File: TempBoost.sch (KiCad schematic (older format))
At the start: 63 parts, among them J1 Conn_01x02, J2 Conn_01x02, Q201 Q_NMOS_GSD, SW101 SW_SPST, T101 3FD-224, U101 DF005S2, U201 MIC2920, U203 UCC27517A, U204 2925, U205 LM2904, U206 TPS1H100, U207 LM1117-5.0, U208 MAX4477

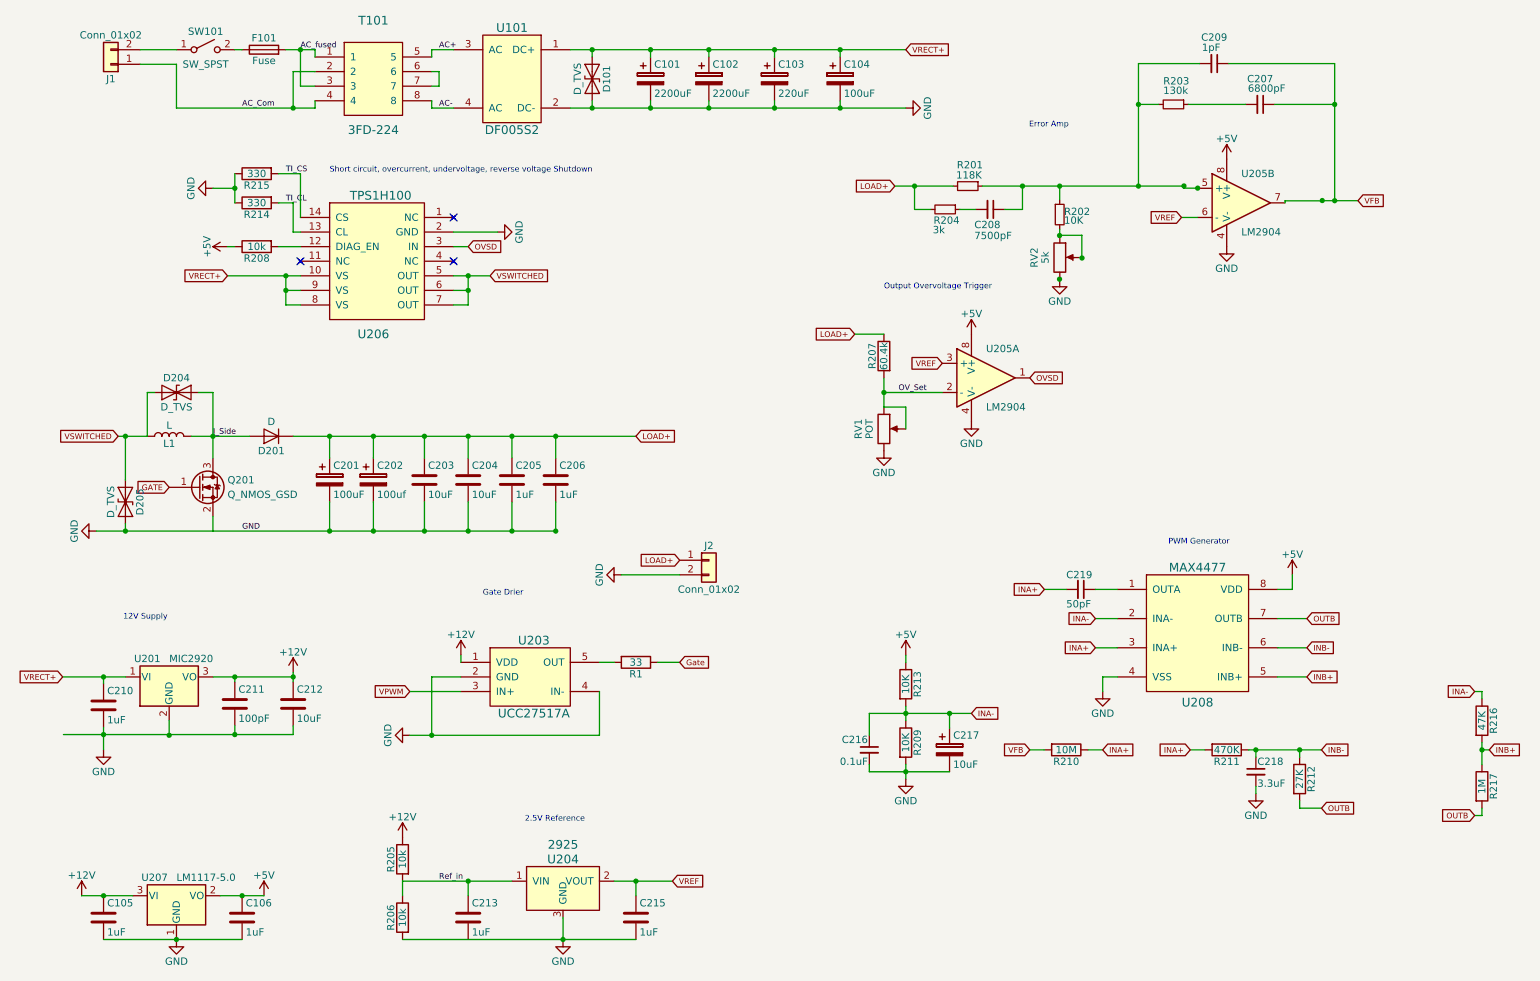
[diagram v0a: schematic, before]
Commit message: Starting Layout
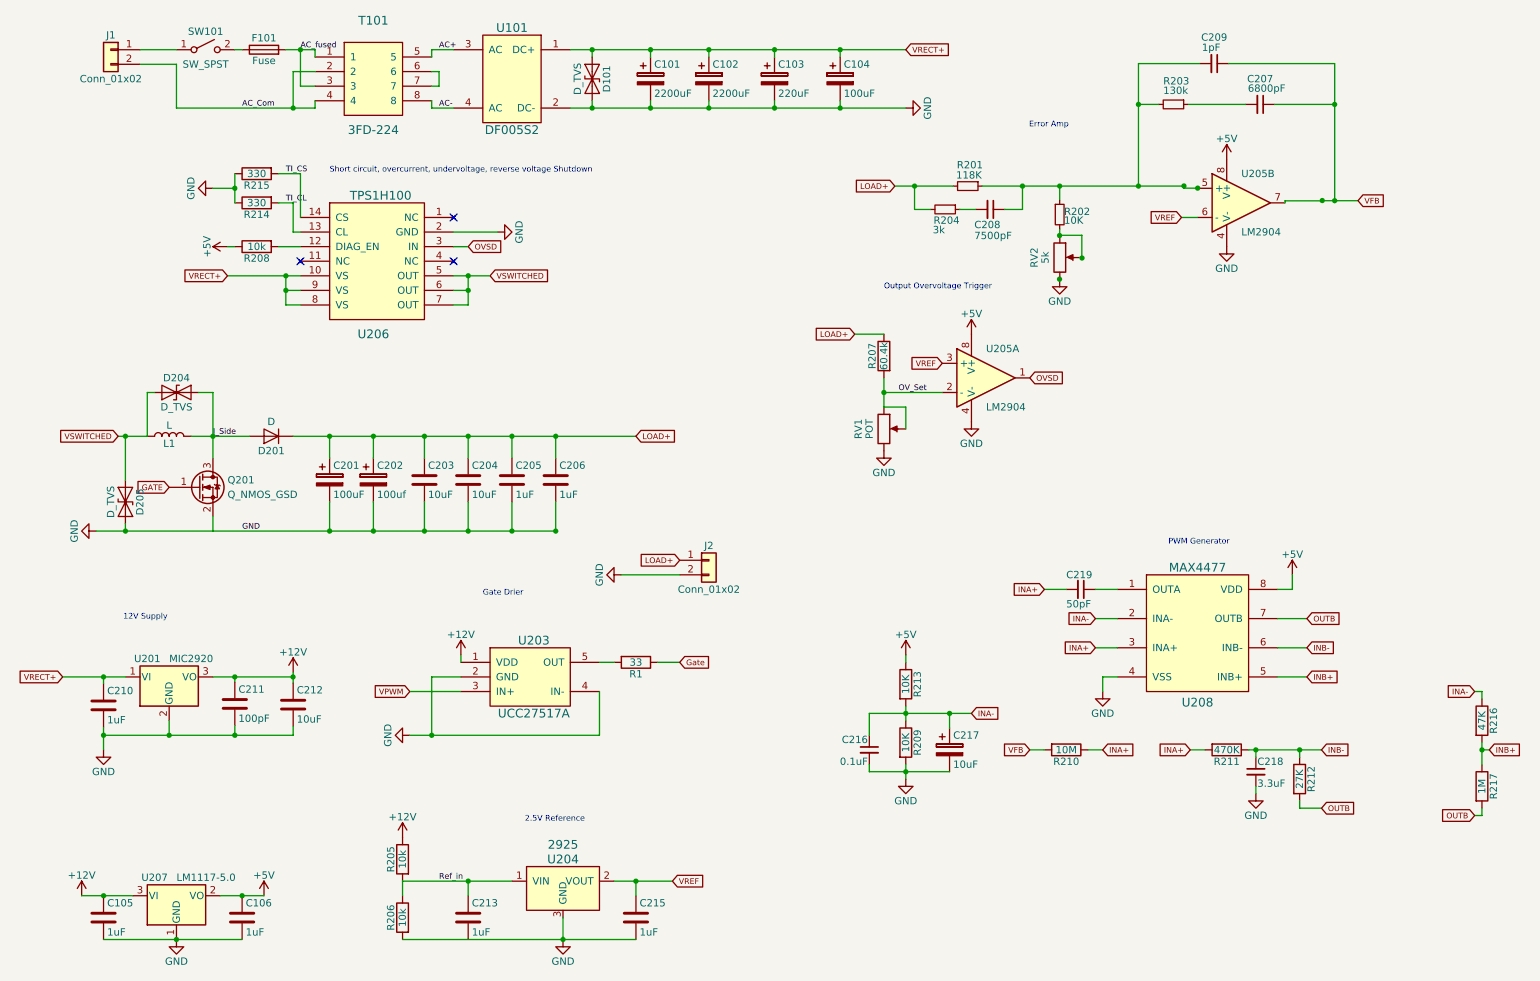
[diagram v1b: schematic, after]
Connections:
- wire segments 166 -> 230
